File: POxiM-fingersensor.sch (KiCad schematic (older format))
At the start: 2 parts

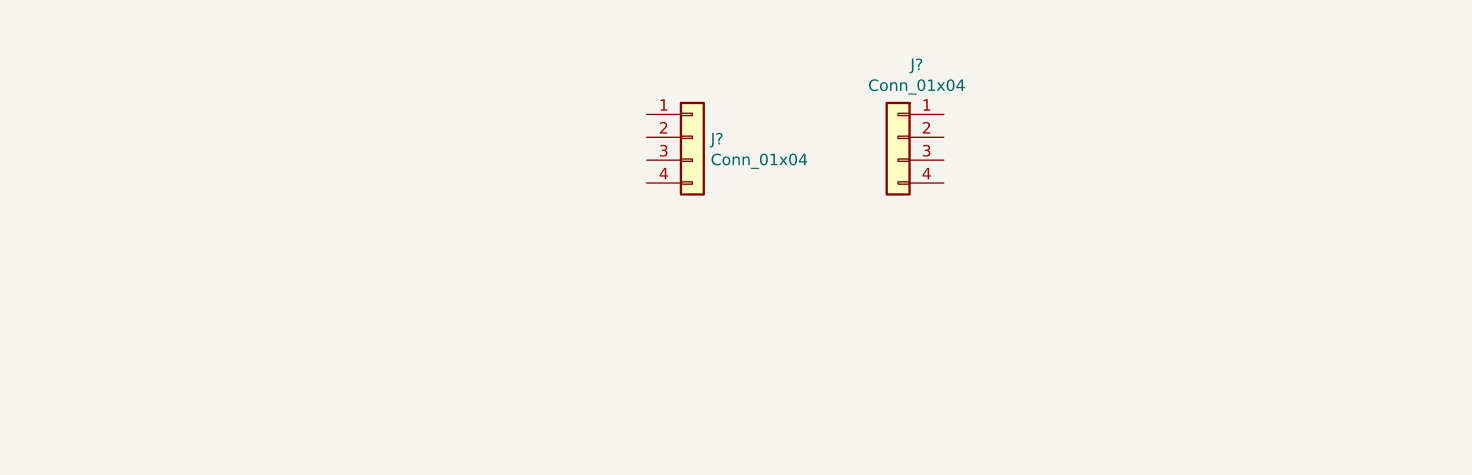
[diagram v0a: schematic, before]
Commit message: Draft scheematic
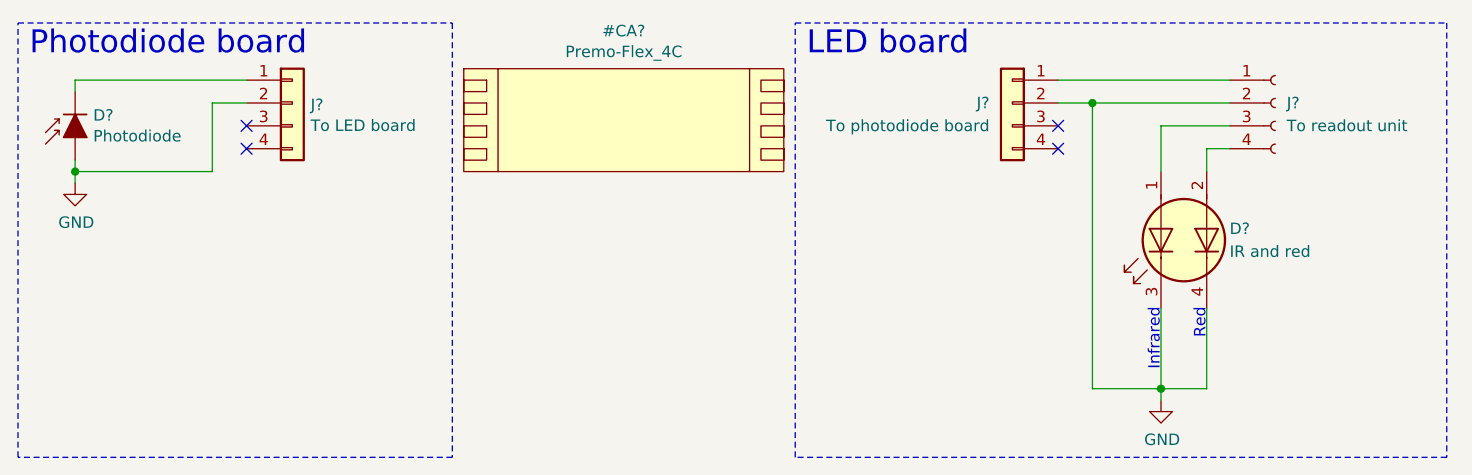
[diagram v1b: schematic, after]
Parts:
- removed J?: Conn_01x04, symbol Connector_Generic:Conn_01x04
- added D?: IR and red, symbol Device:LED_Dual_AACC
- added D?: Photodiode, symbol Device:D_Photo_ALT
- added J?: To LED board, POxiM-uncategorised:Molex_200528-0040_1x04-1MP_P1.00mm_Horizontal, symbol Connector_Generic:Conn_01x04
- added J?: To readout unit, symbol Connector:Conn_01x04_Female
- J?: value Conn_01x04 -> To photodiode board; footprint (none) -> POxiM-uncategorised:Molex_200528-0040_1x04-1MP_P1.00mm_Horizontal; Link (none) -> https://nl.mouser.com/ProductDetail/Molex/200528-0040?qs=sG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; Order number (none) -> 538-200528-0040; Part number (none) -> 2005280040; Supplier (none) -> Mouser
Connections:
- net at J?.1 (Pin_1): now also J?.1 (Pin_1)
- net GND: now reaches J?.2 (Pin_2)
- net GND: now also D?.2 (A), D?.3 (K1), D?.4 (K2), J?.2 (Pin_2), J?.2 (Pin_2)
- new net: D?.1 (K), J?.1 (Pin_1)
- new net: D?.1 (A1), J?.3 (Pin_3)
- new net: D?.2 (A2), J?.4 (Pin_4)
- no-connect marks 0 -> 4
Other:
- note added: "Infrared"
- note added: "LED board"
- note added: "Photodiode board"
- note added: "Red"
- moved on the sheet: J?
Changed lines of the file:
@@
 $Comp
 L Connector_Generic:Conn_01x04 J?
-U 1 1 5EA66398
-P 4800 3400
-F 0 "J?" H 4880 3392 50  0000 L CNN
-F 1 "Conn_01x04" H 4880 3301 50  0000 L CNN
-F 2 "" H 4800 3400 50  0001 C CNN
-F 3 "~" H 4800 3400 50  0001 C CNN
-	1    4800 3400
-	1    0    0    -1
+U 1 1 5EA66BD1
+P 6200 3250
+F 0 "J?" H 6300 3250 50  0000 L CNN
+F 1 "To photodiode board" H 6300 3150 50  0000 L CNN
+F 2 "POxiM-uncategorised:Molex_200528-0040_1x04-1MP_P1.00mm_Horizontal" H 6200 3250 50  0001 C CNN
+F 3 "${KIPRJMOD}/Datasheets/987651-8731.pdf" H 6200 3250 50  0001 C CNN
+F 4 "2005280040" H 6200 3250 50  0001 C CNN "Part number"
+F 5 "538-200528-0040" H 6200 3250 50  0001 C CNN "Order number"
+F 6 "Mouser" H 6200 3250 50  0001 C CNN "Supplier"
+F 7 "" H 6200 3250 50  0001 C CNN "Notes"
+F 8 "https://nl.mouser.com/ProductDetail/Molex/200528-0040?qs=sGAEpiMZZMs7i6cT6ogu4yFxZW78US2djCy2DdTgJmj5TbkKhWqizg%3D%3D" H 6200 3250 50  0001 C CNN "Link"
+	1    6200 3250
+	-1   0    0    -1
 $EndComp
 $Comp
 L Connector_Generic:Conn_01x04 J?
-U 1 1 5EA66BD1
-P 5700 3400
-F 0 "J?" H 5618 3717 50  0000 C CNN
-F 1 "Conn_01x04" H 5618 3626 50  0000 C CNN
-F 2 "" H 5700 3400 50  0001 C CNN
-F 3 "~" H 5700 3400 50  0001 C CNN
-	1    5700 3400
-	-1   0    0    -1
+U 1 1 5EA6A4C1
+P 3050 3250
+F 0 "J?" H 3130 3242 50  0000 L CNN
+F 1 "To LED board" H 3130 3151 50  0000 L CNN
+F 2 "POxiM-uncategorised:Molex_200528-0040_1x04-1MP_P1.00mm_Horizontal" H 3050 3250 50  0001 C CNN
+F 3 "${KIPRJMOD}/Datasheets/987651-8731.pdf" H 3050 3250 50  0001 C CNN
+F 4 "2005280040" H 3050 3250 50  0001 C CNN "Part number"
+F 5 "538-200528-0040" H 3050 3250 50  0001 C CNN "Order number"
+F 6 "Mouser" H 3050 3250 50  0001 C CNN "Supplier"
+F 7 "" H 3050 3250 50  0001 C CNN "Notes"
+F 8 "https://nl.mouser.com/ProductDetail/Molex/200528-0040?qs=sGAEpiMZZMs7i6cT6ogu4yFxZW78US2djCy2DdTgJmj5TbkKhWqizg%3D%3D" H 3050 3250 50  0001 C CNN "Link"
+	1    3050 3250
+	1    0    0    -1
+$EndComp
+Text Notes 6850 4150 3    50   ~ 0
+Infrared
+Text Notes 7050 4150 3    50   ~ 0
+Red
+$Comp
+L Device:D_Photo_ALT D?
+U 1 1 5EA6D793
+P 2100 3400
+F 0 "D?" V 2004 3321 50  0000 R CNN
+F 1 "Photodiode" V 2095 3321 50  0000 R CNN
+F 2 "" H 2050 3400 50  0001 C CNN
+F 3 "~" H 2050 3400 50  0001 C CNN
+	1    2100 3400
+	0    -1   1    0
+$EndComp
+Wire Wire Line
+	2850 3150 2100 3150
+Wire Wire Line
+	2100 3150 2100 3200
+NoConn ~ 2850 3350
+NoConn ~ 2850 3450
+Wire Wire Line
+	2850 3250 2700 3250
+Wire Wire Line
+	2700 3250 2700 3550
+Wire Wire Line
+	2700 3550 2100 3550
+Wire Wire Line
+	2100 3550 2100 3500
+$Comp
+L power:GND #PWR?
+U 1 1 5EA6FEDC
+P 2100 3600
+F 0 "#PWR?" H 2100 3350 50  0001 C CNN
+F 1 "GND" H 2105 3427 50  0000 C CNN
+F 2 "" H 2100 3600 50  0001 C CNN
+F 3 "" H 2100 3600 50  0001 C CNN
+	1    2100 3600
+	1    0    0    -1
+$EndComp
+Wire Wire Line
+	2100 3600 2100 3550
+Connection ~ 2100 3550
+$Comp
+L power:GND #PWR?
+U 1 1 5EA71CA5
+P 6850 4550
+F 0 "#PWR?" H 6850 4300 50  0001 C CNN
+F 1 "GND" H 6855 4377 50  0000 C CNN
+F 2 "" H 6850 4550 50  0001 C CNN
+F 3 "" H 6850 4550 50  0001 C CNN
+	1    6850 4550
+	1    0    0    -1
+$EndComp
+Wire Wire Line
+	6850 4150 6850 4500
+$Comp
+L Device:LED_Dual_AACC D?
+U 1 1 5EA6AA6C
+P 6950 3850
+F 0 "D?" V 6900 3650 50  0000 R CNN
+F 1 "IR and red" V 7000 3650 50  0000 R CNN
+F 2 "" H 6980 3850 50  0001 C CNN
+F 3 "~" H 6980 3850 50  0001 C CNN
+	1    6950 3850
+	0    -1   1    0
+$EndComp
+Wire Wire Line
+	7050 4500 7050 4150
+NoConn ~ 6400 3350
+NoConn ~ 6400 3450
+Wire Wire Line
+	6400 3250 6550 3250
+$Comp
+L Connector:Conn_01x04_Female J?
+U 1 1 5EA73172
+P 7350 3250
+F 0 "J?" H 7400 3250 50  0000 L CNN
+F 1 "To readout unit" H 7400 3150 50  0000 L CNN
+F 2 "" H 7350 3250 50  0001 C CNN
+F 3 "~" H 7350 3250 50  0001 C CNN
+F 4 "1054301204" V 7350 3250 50  0001 C CNN "Part number"
+F 5 "538-105430-1204" V 7350 3250 50  0001 C CNN "Order number"
+F 6 "Mouser" V 7350 3250 50  0001 C CNN "Supplier"
+F 7 "Mouser gold plating, Farnell tin plating" V 7350 3250 50  0001 C CNN "Notes"
+F 8 "https://nl.mouser.com/ProductDetail/Molex/105430-1204?utm_term=1054301204&qs=gZXFycFWdAOazz4rplLXKg%3D%3D&utm_campaign=105430-1204&utm_medium=aggregator&utm_source=findchips&utm_content=Molex" V 7350 3250 50  0001 C CNN "Link"
+F 9 "105430-1104" V 7350 3250 50  0001 C CNN "Part number 2"
+F 10 "3225233" V 7350 3250 50  0001 C CNN "Order number 2"
+F 11 "Farnell" V 7350 3250 50  0001 C CNN "Supplier 2"
+F 12 "https://nl.farnell.com/molex/105430-1104/nano-fit-hdr-smt-ra-sgl-4ckt-tin/dp/3225233?CMP=GRHB-SF-FC" V 7350 3250 50  0001 C CNN "Link 2"
+	1    7350 3250
+	1    0    0    -1
+$EndComp
+Wire Wire Line
+	6850 4500 6850 4550
+Wire Wire Line
+	6400 3150 7150 3150
+Wire Wire Line
+	6850 3550 6850 3350
+Wire Wire Line
+	6850 3350 7150 3350
+Wire Wire Line
+	7050 3550 7050 3450
+Wire Wire Line
+	7050 3450 7150 3450
+Wire Wire Line
+	6850 4500 6550 4500
+Wire Wire Line
+	6550 4500 6550 3250
+Connection ~ 6850 4500
+Connection ~ 6550 3250
+Wire Wire Line
+	6550 3250 7150 3250
+Wire Wire Line
+	6850 4500 7050 4500
+Wire Notes Line
+	5250 2900 8100 2900
+Wire Notes Line
+	8100 2900 8100 4800
+Wire Notes Line
+	8100 4800 5250 4800
+Wire Notes Line
+	5250 4800 5250 2900
+Wire Notes Line
+	3750 2900 3750 4800
+Wire Notes Line
+	3750 4800 1850 4800
+Wire Notes Line
+	1850 4800 1850 2900
+Wire Notes Line
+	1850 2900 3750 2900
+Text Notes 5300 3050 0    100  ~ 0
+LED board
+Text Notes 1900 3050 0    100  ~ 0
+Photodiode board
+$Comp
+L POxiM-mechanical:Premo-Flex_4C #CA?
+U 1 1 5EA7B2D1
+P 4500 3300
+F 0 "#CA?" H 4500 3665 50  0000 C CNN
+F 1 "Premo-Flex_4C" H 4500 3574 50  0000 C CNN
+F 2 "" H 4850 3550 50  0001 C CNN
+F 3 "" H 4850 3550 50  0001 C CNN
+	1    4500 3300
+	1    0    0    -1
 $EndComp
 $EndSCHEMATC
